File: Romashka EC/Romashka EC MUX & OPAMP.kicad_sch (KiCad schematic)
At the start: 31 parts, among them U4 OPA2365, U5 4052, U6 OPA2365, U7 4052

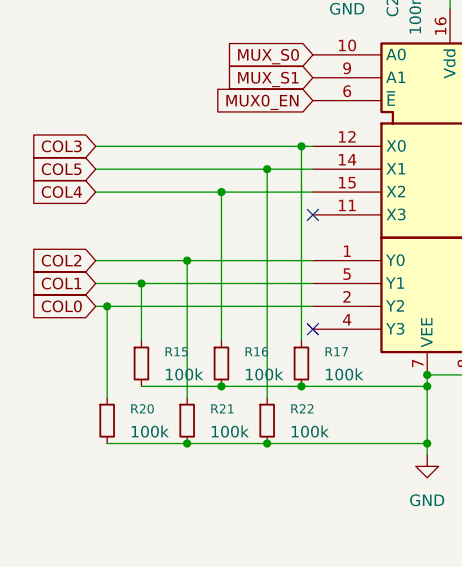
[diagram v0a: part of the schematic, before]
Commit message: 21.04.2026: footprints
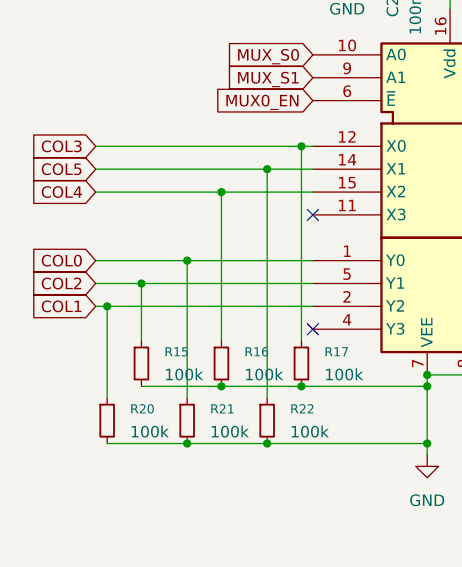
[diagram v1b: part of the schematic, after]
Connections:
- net COL0: now also R21.1, U5.1 (Y0); no longer R20.1, U5.2 (Y2)
- net COL1: now also R20.1, U5.2 (Y2); no longer R15.1, U5.5 (Y1)
- net COL2: now also R15.1, U5.5 (Y1); no longer R21.1, U5.1 (Y0)
